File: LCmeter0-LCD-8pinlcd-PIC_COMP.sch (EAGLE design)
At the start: 34 parts, among them IC1 PIC16F876A-X/SP-COMP-B-A/V, J1 HD44780, J2 PIC-UART, J3 PIC-ICSPICSP, K2 DS2Y, Q1 20MHz, T1 BC547, X1 FREQ, X2 L/C

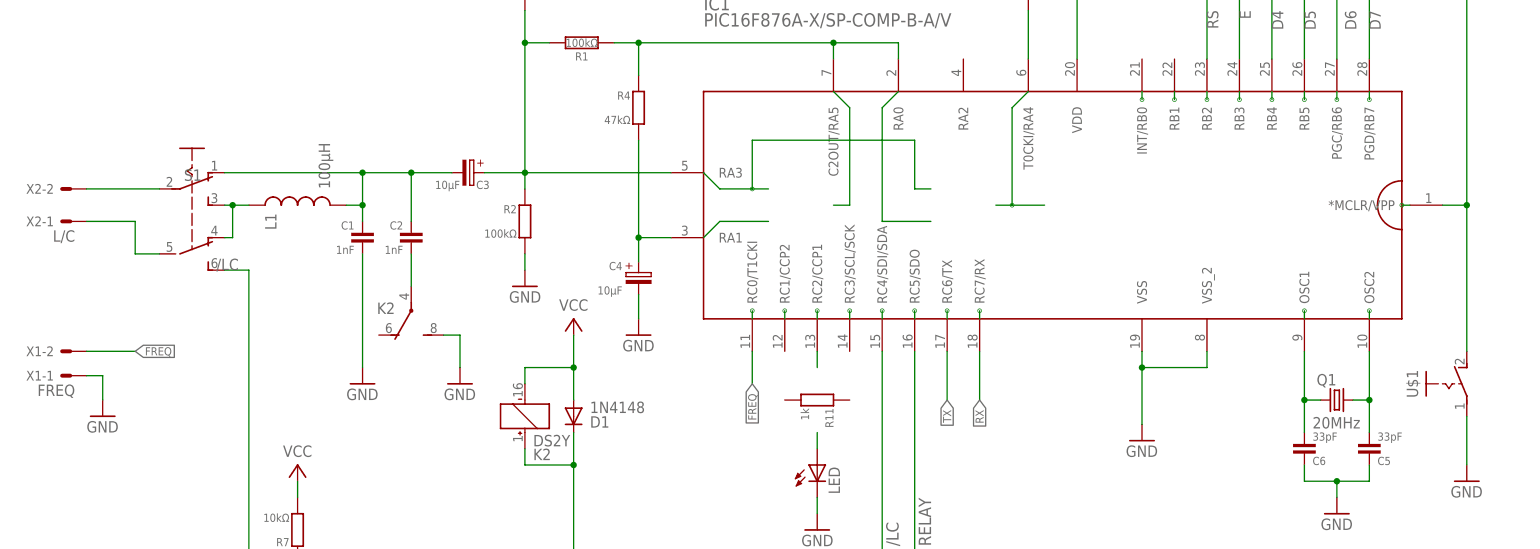
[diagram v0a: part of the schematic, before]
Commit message: ...
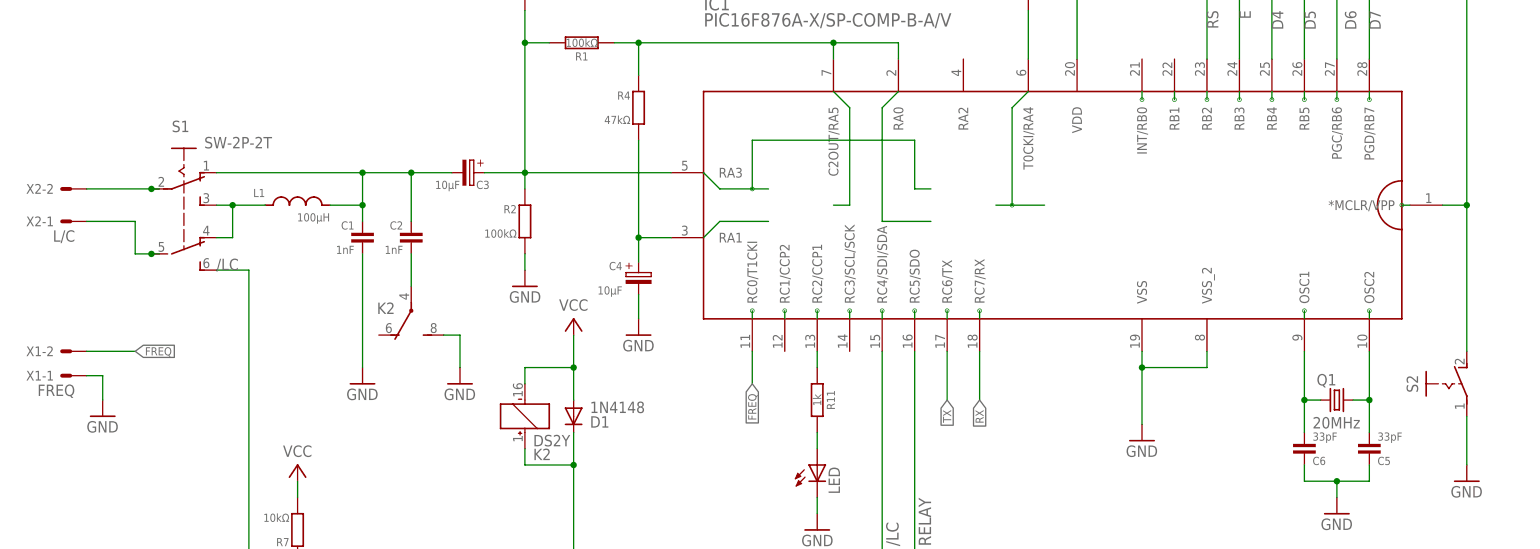
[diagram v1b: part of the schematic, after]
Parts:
- L1: value 100μH -> 100µH; device r:L02/5 -> l:L-SHORT02/5
- R11: device r:R0202/5 -> r:R-H0202/5
- S1: value SL-SW-2P-2T -> SW-2P-2T; device sw:SL-SW-2P-2T -> sw:SW-2P-2T
- renumbered U$1 to S2
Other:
- moved on the sheet: S1
